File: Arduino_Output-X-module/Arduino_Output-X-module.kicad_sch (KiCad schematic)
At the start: 12 parts, among them J1 Screw_Terminal_01x04, J2 Screw_Terminal_01x08, Q1 IRF540N, U1 MAX485_MODULE_5V_LOGIC_TLL_TO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, U2 LM2596S-5

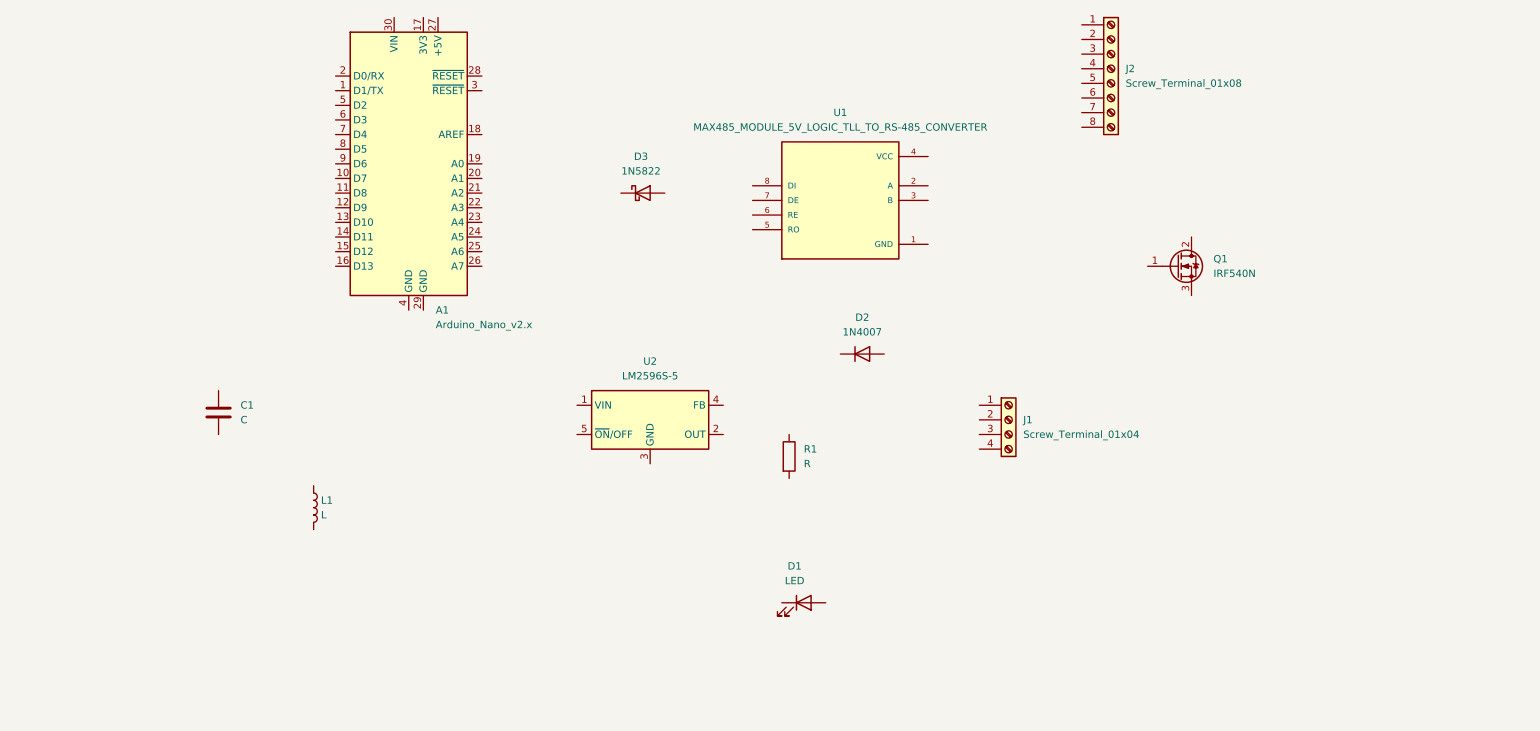
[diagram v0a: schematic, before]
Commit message: finishhed schematic
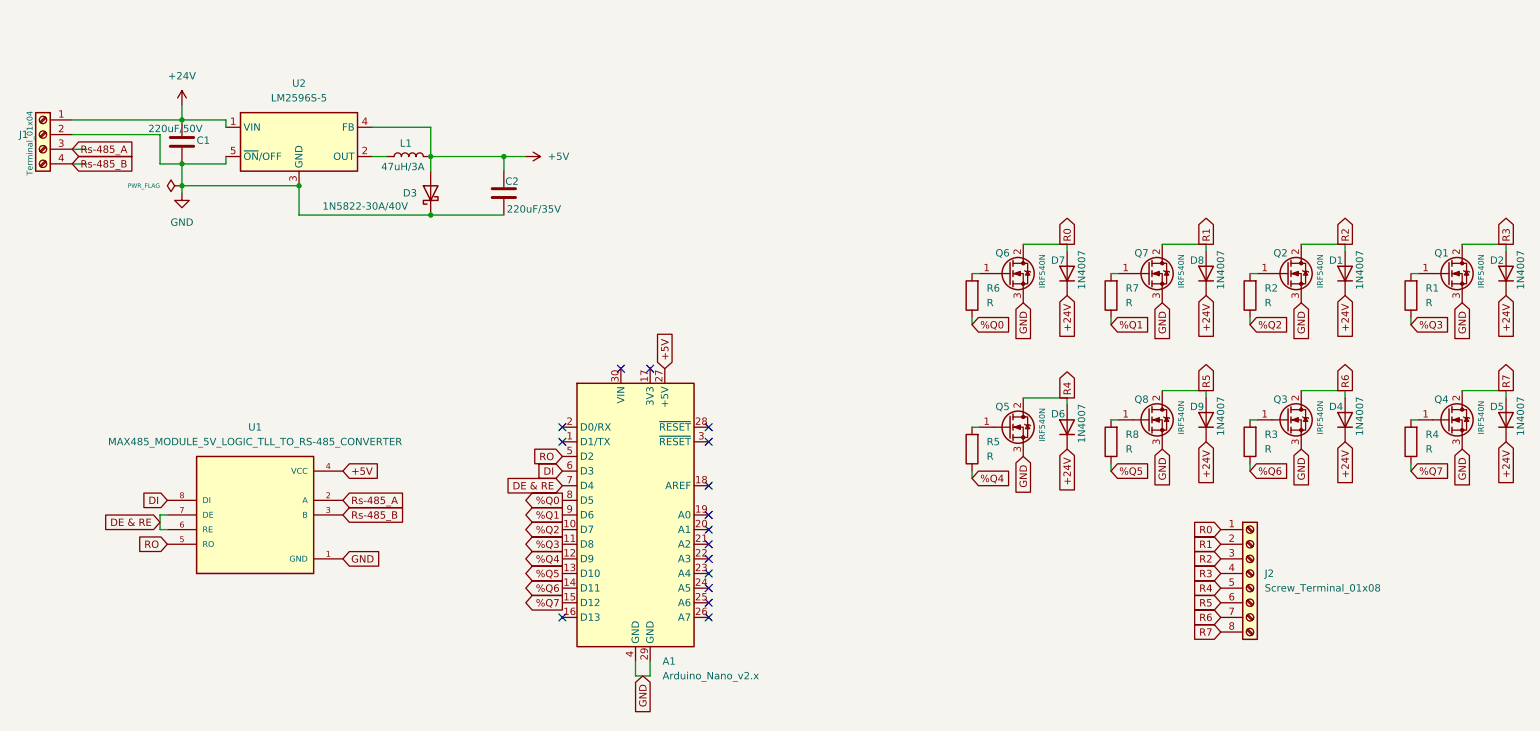
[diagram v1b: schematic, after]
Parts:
- removed D1: LED, symbol Device:LED
- added C2: 220uF/35V, symbol Device:C
- added D1, D4, D5, D6, D7, D8, D9: 1N4007, Diode_THT:D_DO-41_SOD81_P10.16mm_Horizontal, symbol Diode:1N4007
- added Q2, Q3, Q4, Q5, Q6, Q7, Q8: IRF540N, Package_TO_SOT_THT:TO-220-3_Vertical, symbol Transistor_FET:IRF540N
- added R2, R3, R4, R5, R6, R7, R8: R, symbol Device:R
- C1: value C -> 220uF/50V
- D3: value 1N5822 -> 1N5822-30A/40V
- J1: value Screw_Terminal_01x04 -> Terminal_01x04
- L1: value L -> 47uH/3A
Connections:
- net %Q2: now reaches A1.10 (D7)
- net %Q2: now also R2.1
- net %Q3: now reaches A1.11 (D8)
- net %Q3: now also R1.1
- net %Q4: now reaches A1.12 (D9)
- net %Q4: now also R5.1
- net %Q5: now reaches A1.13 (D10)
- net %Q5: now also R8.1
- net %Q6: now reaches A1.14 (D11)
- net %Q6: now also R3.1
- net %Q7: now reaches A1.15 (D12)
- net %Q7: now also R4.1
- net +5V: now reaches A1.27 (+5V)
- net +5V: now also D3.2 (A), L1.2, U1.4 (VCC), U2.4 (FB), C2.1
- net GND: now reaches A1.29 (GND)
- net GND: now also A1.4 (GND), C1.2, D3.1 (K), J1.2 (Pin_2), Q1.3 (S), U1.1 (GND), U2.3 (GND), U2.5 (~{ON}/OFF), C2.2, Q2.3 (S), Q3.3 (S), Q4.3 (S), Q5.3 (S), Q6.3 (S), Q7.3 (S), Q8.3 (S)
- net RO: now reaches A1.5 (D2)
- net RO: now also U1.5 (RO)
- net DI: now reaches A1.6 (D3)
- net DI: now also U1.8 (DI)
- net DE & RE: now reaches A1.7 (D4)
- net DE & RE: now also U1.6 (RE), U1.7 (DE)
- net %Q0: now reaches A1.8 (D5)
- net %Q0: now also R6.1
- net %Q1: now reaches A1.9 (D6)
- net %Q1: now also R7.1
- net +24V: now reaches D2.1 (K)
- net +24V: now also C1.1, J1.1 (Pin_1), U2.1 (VIN), D1.1 (K), D4.1 (K), D5.1 (K), D6.1 (K), D7.1 (K), D8.1 (K), D9.1 (K)
- net R3: now reaches D2.2 (A)
- net R3: now also J2.4 (Pin_4), Q1.2 (D)
- net at U2.2 (OUT): now also L1.1
- net Rs-485_A: now reaches J1.3 (Pin_3)
- net Rs-485_A: now also U1.2 (A)
- net Rs-485_B: now reaches J1.4 (Pin_4)
- net Rs-485_B: now also U1.3 (B)
- net R0: now reaches J2.1 (Pin_1)
- net R0: now also D7.2 (A), Q6.2 (D)
- net R1: now reaches J2.2 (Pin_2)
- net R1: now also D8.2 (A), Q7.2 (D)
- net R2: now reaches J2.3 (Pin_3)
- net R2: now also D1.2 (A), Q2.2 (D)
- net R4: now reaches J2.5 (Pin_5)
- net R4: now also D6.2 (A), Q5.2 (D)
- net R5: now reaches J2.6 (Pin_6)
- net R5: now also D9.2 (A), Q8.2 (D)
- net R6: now reaches J2.7 (Pin_7)
- net R6: now also D4.2 (A), Q3.2 (D)
- net R7: now reaches J2.8 (Pin_8)
- net R7: now also D5.2 (A), Q4.2 (D)
- net at R1.2: now also Q1.1 (G)
- new net: Q8.1 (G), R8.2
- new net: Q3.1 (G), R3.2
- new net: Q7.1 (G), R7.2
- new net: Q2.1 (G), R2.2
- new net: Q6.1 (G), R6.2
- new net: Q5.1 (G), R5.2
- new net: Q4.1 (G), R4.2
- no-connect marks 0 -> 16
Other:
- moved on the sheet: A1, C1, D2, D3, J1, J2, L1, Q1, R1, U1, U2

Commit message: finishhed assigninf footprints
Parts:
- C1: footprint (none) -> Capacitor_THT:CP_Radial_D10.0mm_P5.00mm
- C2: footprint (none) -> Capacitor_THT:CP_Radial_D8.0mm_P3.80mm
- J1: footprint (none) -> Connector_IDC:IDC-Header_2x04_P2.54mm_Horizontal
- J2: footprint (none) -> TerminalBlock_Phoenix:TerminalBlock_Phoenix_MKDS-1,5-12_1x12_P5.00mm_Horizontal
- L1: footprint (none) -> Inductor_THT:L_Radial_D10.0mm_P5.00mm_Fastron_07M
- R1, R2, R3, R4, R5, R6, R7, R8: footprint (none) -> Resistor_THT:R_Axial_DIN0207_L6.3mm_D2.5mm_P2.54mm_Vertical
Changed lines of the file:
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@@
 			)
 		)
-		(property "Footprint" ""
+		(property "Footprint" "Connector_IDC:IDC-Header_2x04_P2.54mm_Horizontal"
 			(at 21.59 57.15 0)
 			(effects
@@
 			)
 		)
-		(property "Footprint" ""
+		(property "Footprint" "TerminalBlock_Phoenix:TerminalBlock_Phoenix_MKDS-1,5-12_1x12_P5.00mm_Horizontal"
 			(at 231.14 133.35 0)
 			(effects
@@
 			)
 		)
-		(property "Footprint" ""
+		(property "Footprint" "Capacitor_THT:CP_Radial_D8.0mm_P3.80mm"
 			(at 102.5652 71.12 0)
 			(effects
@@
 			)
 		)
-		(property "Footprint" ""
+		(property "Footprint" "Capacitor_THT:CP_Radial_D10.0mm_P5.00mm"
 			(at 46.6852 62.23 0)
 			(effects
@@
 			)
 		)
-		(property "Footprint" ""
+		(property "Footprint" "Resistor_THT:R_Axial_DIN0207_L6.3mm_D2.5mm_P2.54mm_Vertical"
 			(at 260.858 85.09 90)
 			(effects
@@
 			)
 		)
-		(property "Footprint" ""
+		(property "Footprint" "Resistor_THT:R_Axial_DIN0207_L6.3mm_D2.5mm_P2.54mm_Vertical"
 			(at 232.918 110.49 90)
 			(effects
@@
 			)
 		)
-		(property "Footprint" ""
+		(property "Footprint" "Resistor_THT:R_Axial_DIN0207_L6.3mm_D2.5mm_P2.54mm_Vertical"
 			(at 208.788 110.49 90)
 			(effects
@@
 			)
 		)
-		(property "Footprint" ""
+		(property "Footprint" "Resistor_THT:R_Axial_DIN0207_L6.3mm_D2.5mm_P2.54mm_Vertical"
 			(at 208.788 85.09 90)
 			(effects
@@
 			)
 		)
-		(property "Footprint" ""
+		(property "Footprint" "Resistor_THT:R_Axial_DIN0207_L6.3mm_D2.5mm_P2.54mm_Vertical"
 			(at 184.658 85.09 90)
 			(effects
@@
 			)
 		)
-		(property "Footprint" ""
+		(property "Footprint" "Resistor_THT:R_Axial_DIN0207_L6.3mm_D2.5mm_P2.54mm_Vertical"
 			(at 232.918 85.09 90)
 			(effects
@@
 			)
 		)
-		(property "Footprint" ""
+		(property "Footprint" "Inductor_THT:L_Radial_D10.0mm_P5.00mm_Fastron_07M"
 			(at 85.09 60.96 0)
 			(effects
@@
 			)
 		)
-		(property "Footprint" ""
+		(property "Footprint" "Resistor_THT:R_Axial_DIN0207_L6.3mm_D2.5mm_P2.54mm_Vertical"
 			(at 184.658 111.76 90)
 			(effects
@@
 			)
 		)
-		(property "Footprint" ""
+		(property "Footprint" "Resistor_THT:R_Axial_DIN0207_L6.3mm_D2.5mm_P2.54mm_Vertical"
 			(at 260.858 110.49 90)
 			(effects
